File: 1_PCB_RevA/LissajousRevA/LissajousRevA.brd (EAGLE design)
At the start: 100 x 80 mm, 87 parts, among them U101 LM348D, U201 LM348D, U401 LM348D

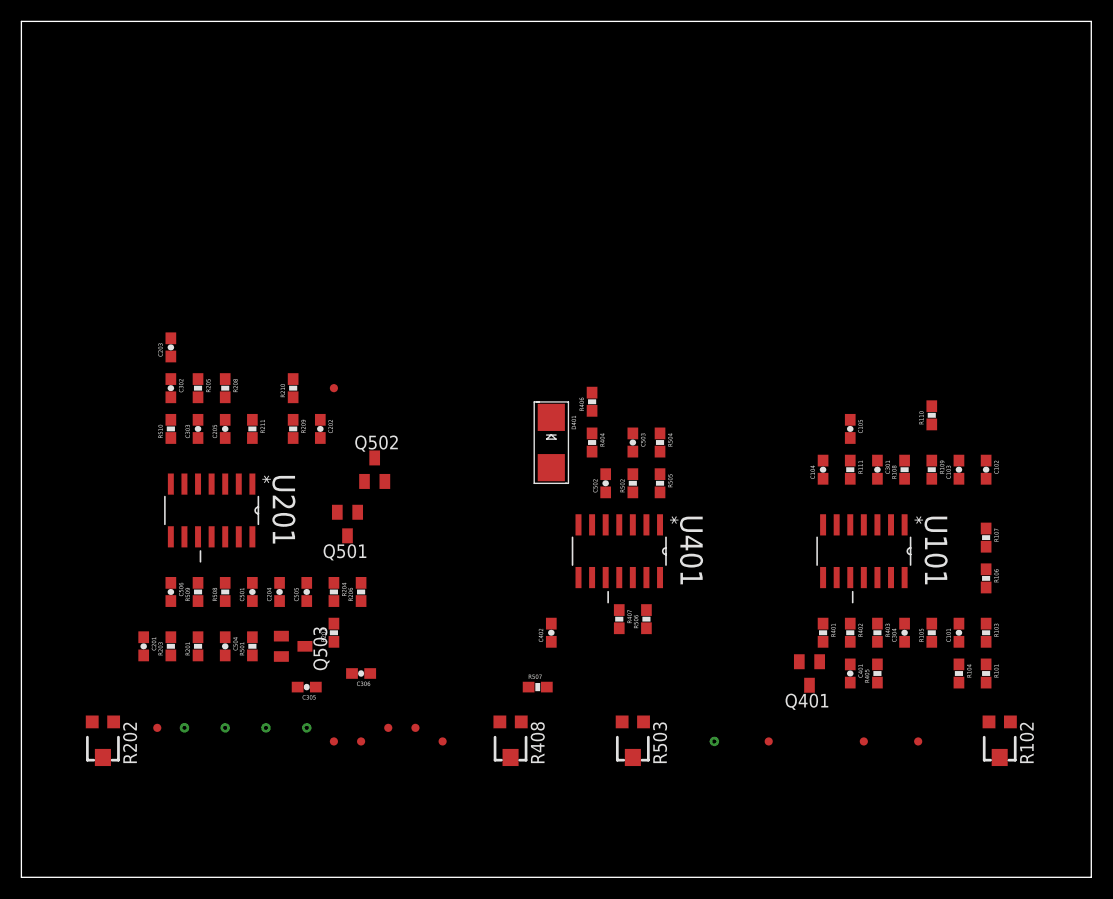
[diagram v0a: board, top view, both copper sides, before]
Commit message: lots of routing and another net fix
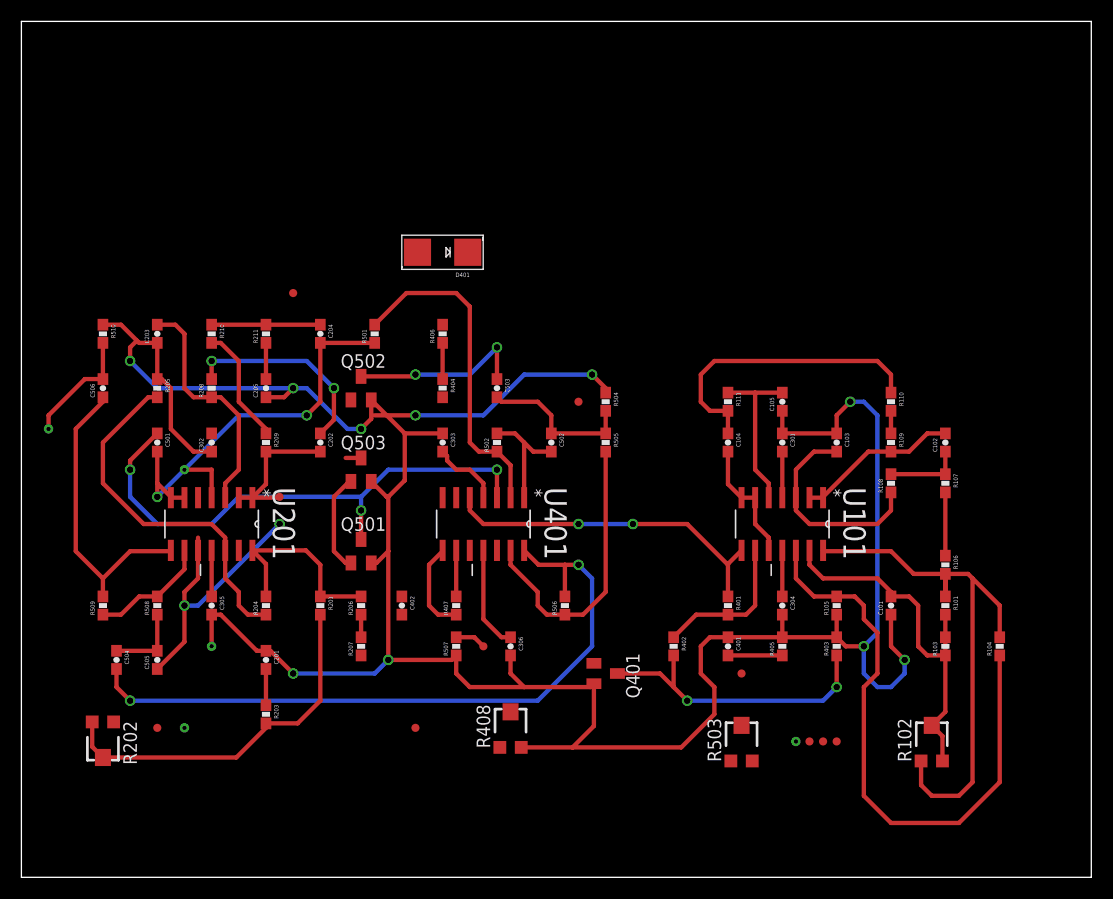
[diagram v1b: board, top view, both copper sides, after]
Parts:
- moved TP305 36.9 mm to (2.54, 41.9)
- moved TP501 35.3 mm to (52.1, 44.5)
- moved R501 31.4 mm to (33.0, 50.8)
- moved TP401 28.7 mm to (67.3, 19.1)
- moved TP301 25.3 mm to (15.2, 38.1)
- moved C204 24.4 mm to (27.9, 50.8), turned to 270 degrees
- moved TP202 24.1 mm to (24.1, 35.6)
- moved C303 22.9 mm to (39.4, 40.6), turned to 270 degrees
- moved D401 20.5 mm to (39.4, 58.4), turned to 180 degrees
- moved C506 20.1 mm to (7.62, 45.7), turned to 90 degrees
- moved Q401 19.0 mm to (54.6, 19.1), turned to 270 degrees
- moved Q503 17.7 mm to (31.8, 38.1), turned to 0 degrees
- moved C501 16.6 mm to (12.7, 40.6), turned to 270 degrees
- moved R402 16.6 mm to (61.0, 21.6)
- moved TP502 16.6 mm to (43.2, 21.6)
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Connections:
- removed net N$41: C504.2
- net N$39: now also C504.2
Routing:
- net 0V: track 0.00 -> 259.7 mm, vias 0 -> 10
- net N$39: track 0.00 -> 65.5 mm, vias 0 -> 2
- net N$2: track 0.00 -> 56.0 mm
- net N$7: track 0.00 -> 52.5 mm
- net N$20: track 0.00 -> 51.0 mm, vias 0 -> 3
- net SINEGEN2: track 0.00 -> 36.9 mm, vias 0 -> 2
- net N$24: track 0.00 -> 34.5 mm
- net N$9: track 0.00 -> 33.9 mm
- net VIEW1: track 0.00 -> 32.3 mm, vias 0 -> 2
- net N$26: track 0.00 -> 31.1 mm
- net N$46: track 0.00 -> 28.2 mm
- net N$12: track 0.00 -> 28.1 mm
- net N$31: track 0.00 -> 28.0 mm, vias 0 -> 2
- net N$45: track 0.00 -> 27.3 mm, vias 0 -> 2
- net N$37: track 0.00 -> 26.9 mm
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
